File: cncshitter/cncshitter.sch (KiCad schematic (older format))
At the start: 54 parts, among them J1 24V_IN, J2 5V_IN, J3 DB25_Male_MountingHoles, J4 SPINDLE_PWM_ENC, J5 SPINDLE_ENABLE, J6 EMERGENCY_PROBE_ENABLE, J7 AXIS_XYZ, K1 SANYOU_SRD_Form_C, K2 SANYOU_SRD_Form_C, U1 EMERGENCY, U10 AXIS_Y_STEP, U11 AXIS_Z_DIR, U12 AXIS_Z_STEP, U2 PROBE, U3 ENABLE, U4 SPINDLE_PWM, U5 SPINDLE_ENC, U6 SPINDLE_ENABLE, U7 AXIS_X_DIR, U8 AXIS_X_STEP, U9 AXIS_Y_DIR

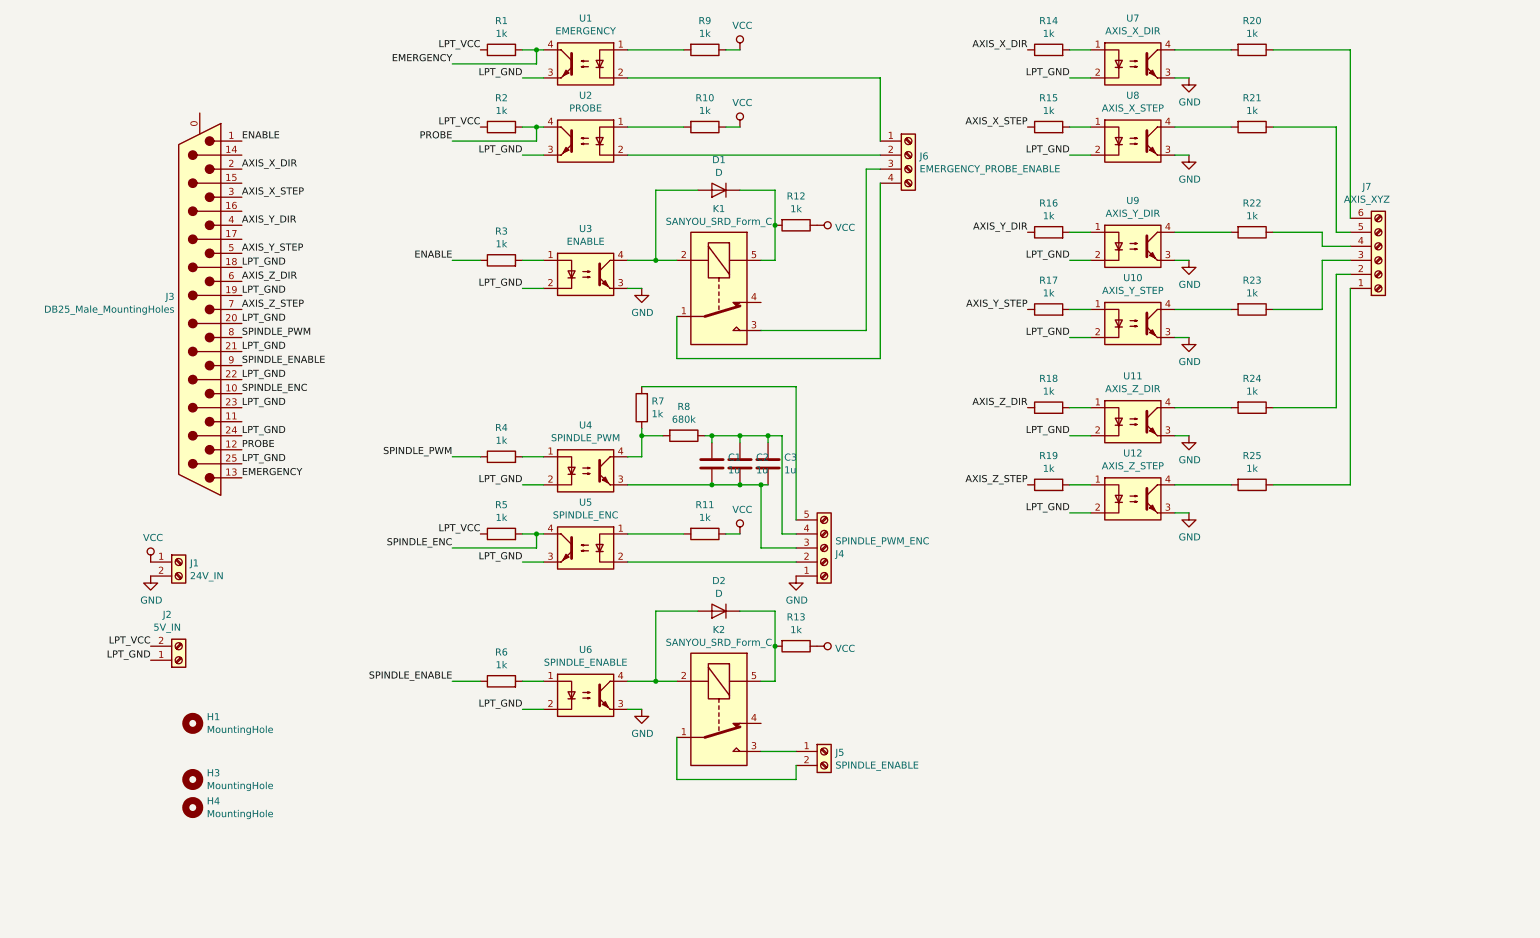
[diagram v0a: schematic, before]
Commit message: v5
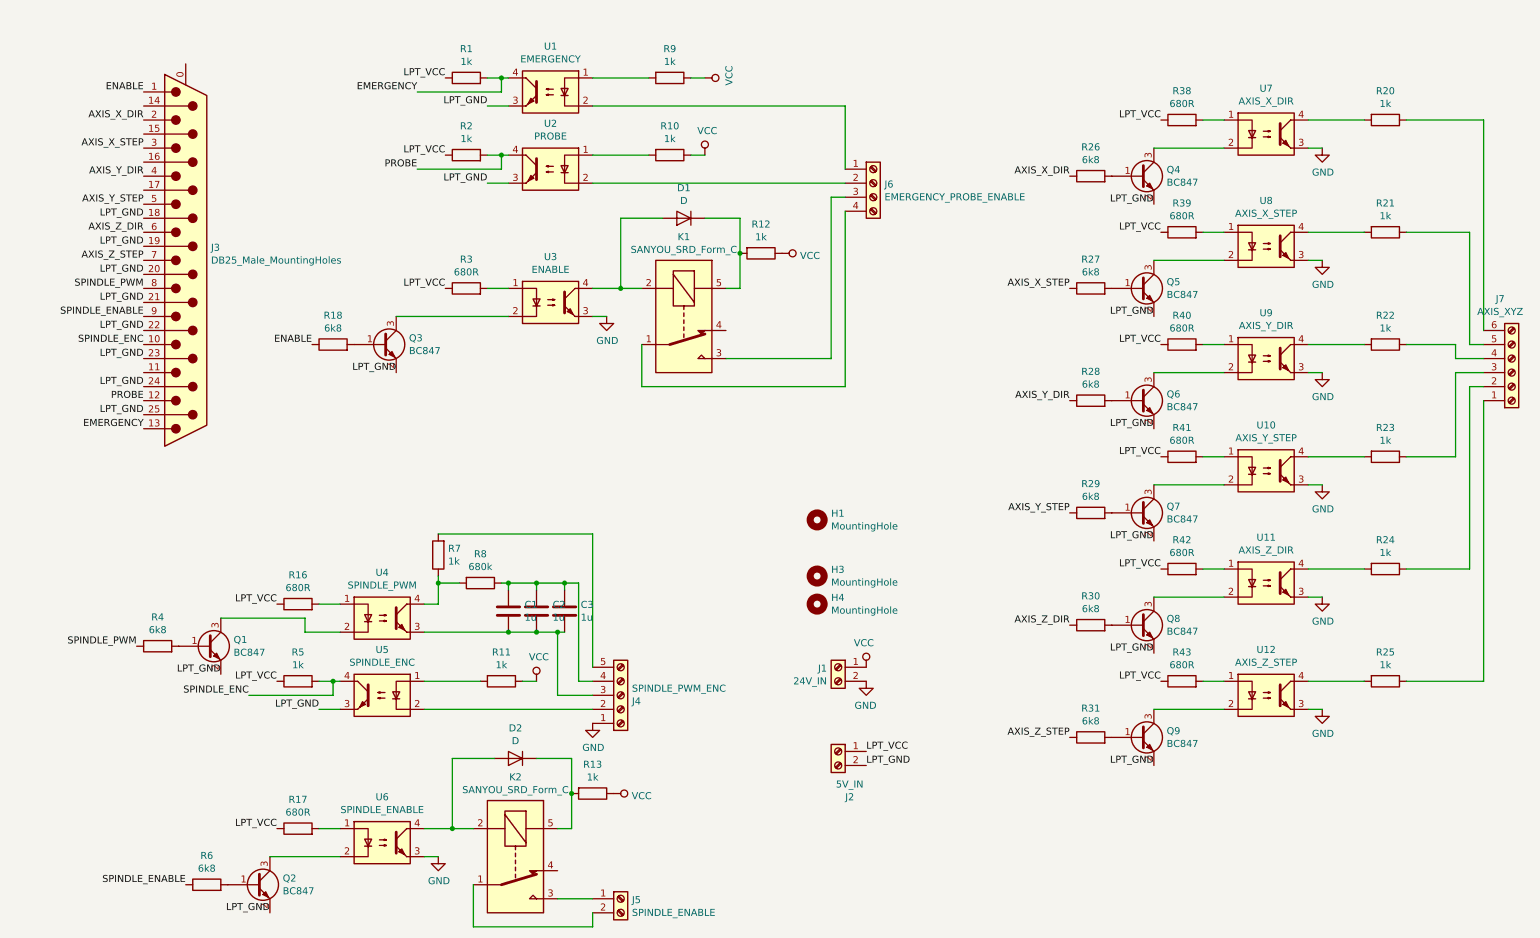
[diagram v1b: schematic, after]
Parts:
- removed R14, R15, R19: 1k, Resistor_SMD:R_1206_3216Metric_Pad1.42x1.75mm_HandSolder, symbol Device:R
- added Q1, Q2, Q3, Q4, Q5, Q6, Q7, Q8, Q9: BC847, Package_TO_SOT_SMD:SOT-23, symbol Transistor_BJT:BC847
- added R26, R27, R28, R29, R30, R31: 6k8, Resistor_SMD:R_1206_3216Metric_Pad1.42x1.75mm_HandSolder, symbol Device:R
- added R38, R39, R40, R41, R42, R43: 680R, Resistor_SMD:R_1206_3216Metric_Pad1.42x1.75mm_HandSolder, symbol Device:R
- R16, R17, R3: value 1k -> 680R
- R18, R4, R6: value 1k -> 6k8
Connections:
- net AXIS_X_DIR: now also R26.1
- net AXIS_X_STEP: now also R27.1
- net AXIS_Y_DIR: now also R28.1; no longer R16.1
- net AXIS_Y_STEP: now also R29.1; no longer R17.1
- net AXIS_Z_DIR: now also R30.1; no longer R18.1
- net AXIS_Z_STEP: now also R31.1
- net ENABLE: now also R18.1; no longer R3.1
- net LPT_GND: now also J2.2 (Pin_2), Q1.2 (E), Q2.2 (E), Q3.2 (E), Q4.2 (E), Q5.2 (E), Q6.2 (E), Q7.2 (E), Q8.2 (E), Q9.2 (E); no longer J2.1 (Pin_1), U10.2, U11.2, U12.2, U3.2, U4.2, U6.2, U7.2, U8.2, U9.2
- net LPT_VCC: now also J2.1 (Pin_1), R16.1, R17.1, R3.1, R38.1, R39.1, R40.1, R41.1, R42.1, R43.1; no longer J2.2 (Pin_2)
- net at U7.1: now also R38.2
- net at U8.1: now also R39.2
- net at U9.1: now also R40.2; no longer R16.2
- net at U10.1: now also R41.2; no longer R17.2
- net at U11.1: now also R42.2; no longer R18.2
- net at U12.1: now also R43.2
- net at U4.1: now also R16.2; no longer R4.2
- net at U6.1: now also R17.2; no longer R6.2
- new net: Q4.3 (C), U7.2
- new net: Q5.3 (C), U8.2
- new net: Q6.3 (C), U9.2
- new net: Q7.3 (C), U10.2
- new net: Q8.3 (C), U11.2
- new net: Q9.3 (C), U12.2
- new net: Q3.1 (B), R18.2
- new net: Q3.3 (C), U3.2
- new net: Q1.3 (C), U4.2
- new net: Q1.1 (B), R4.2
- new net: Q2.3 (C), U6.2
- new net: Q2.1 (B), R6.2
- new net: Q4.1 (B), R26.2
- new net: Q5.1 (B), R27.2
- new net: Q6.1 (B), R28.2
- new net: Q8.1 (B), R30.2
- new net: Q7.1 (B), R29.2
- new net: Q9.1 (B), R31.2
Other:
- moved on the sheet: C1, C2, C3, D1, D2, H1, H3, H4, J1, J2, J3, J4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
